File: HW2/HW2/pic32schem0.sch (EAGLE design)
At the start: 21 parts, among them J3 USB-MB-H

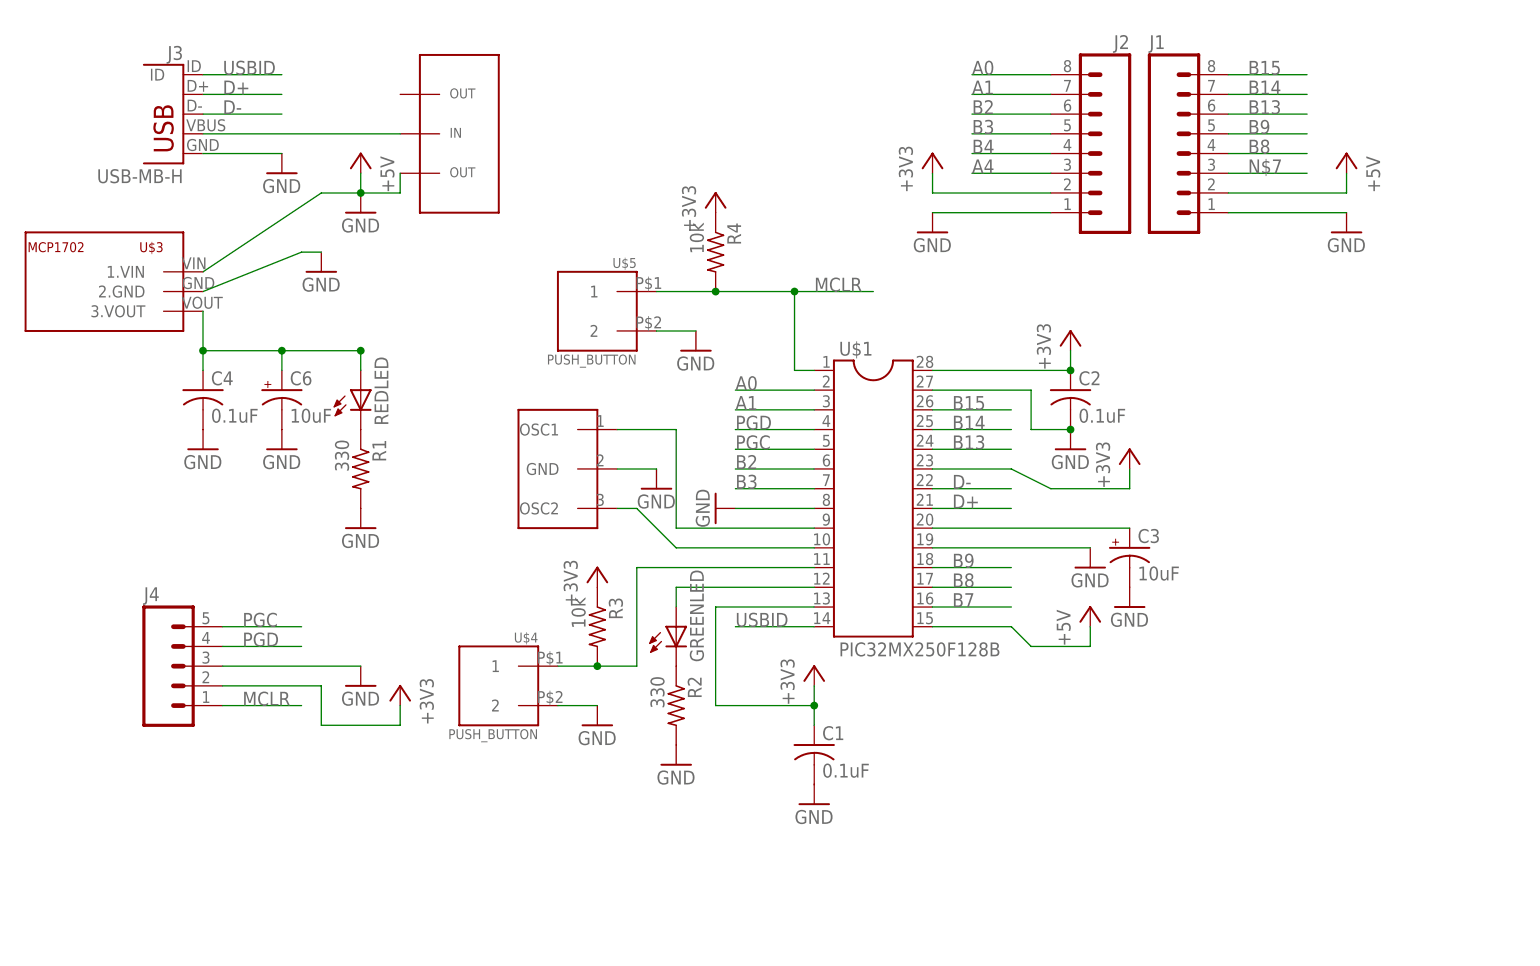
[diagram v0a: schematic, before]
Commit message: Finished pcb, quite a few errors
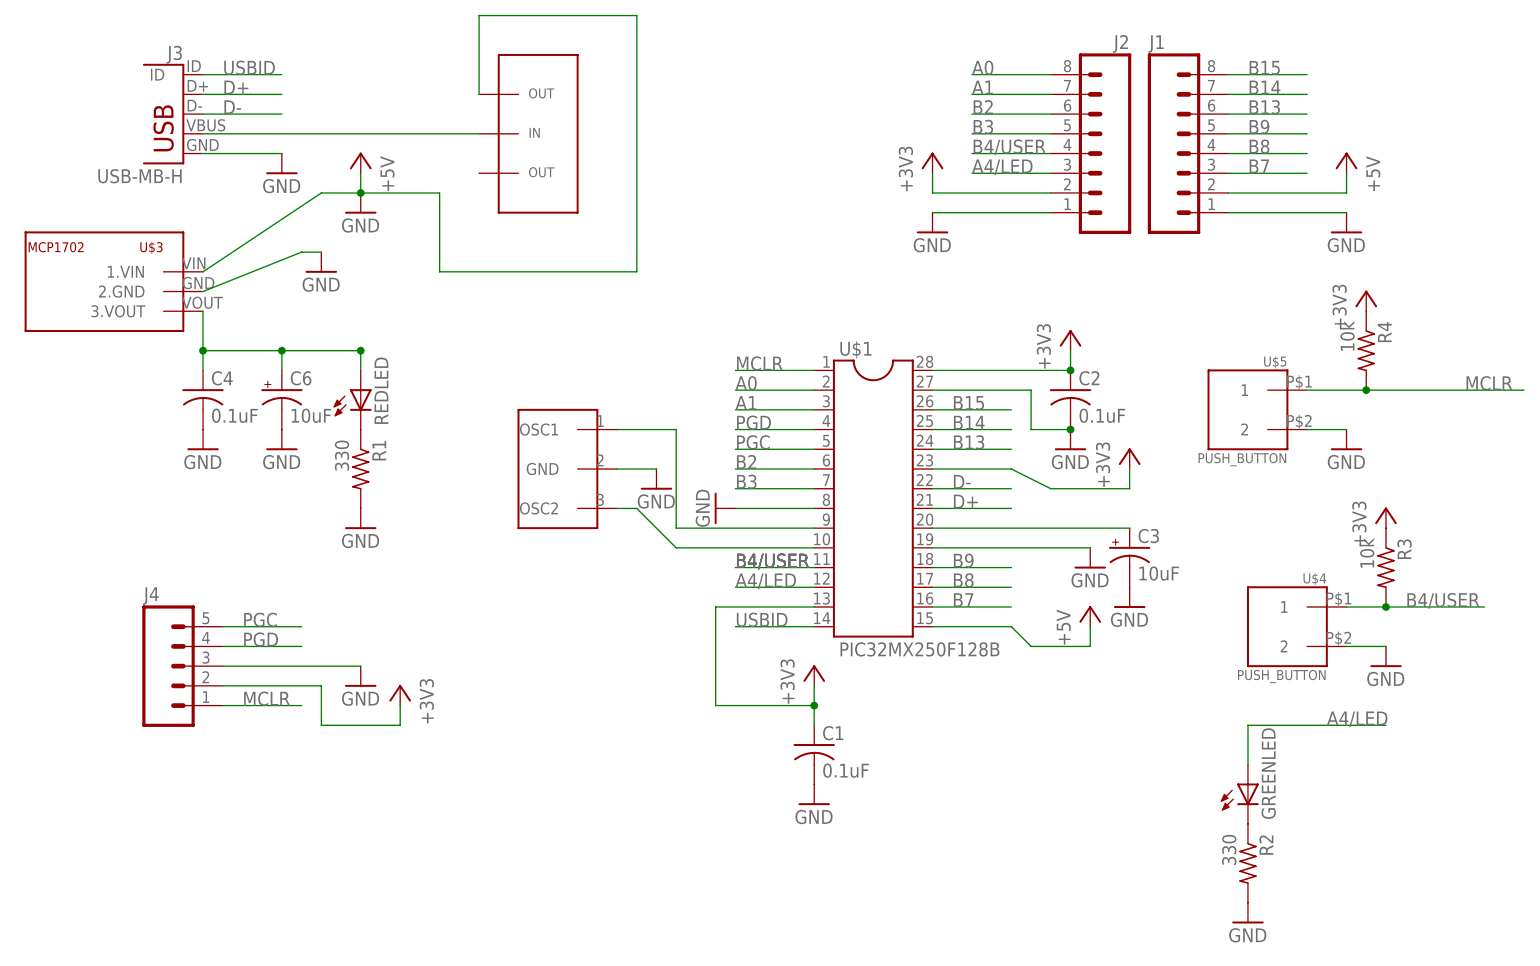
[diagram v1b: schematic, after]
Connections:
- removed net A1/LED: GREENLED.A, U$1.12.SOSCO/RPA4/T1CK/CTED9/PMA1/RA4
- removed net A4: J2.3
- removed net B4: J2.4
- removed net N$7: J1.3
- new net A4/LED: GREENLED.A, J2.3, U$1.12.SOSCO/RPA4/T1CK/CTED9/PMA1/RA4
- net B4/USER: now also J2.4
- net B7: now also J1.3
- net GND: now also U$2.3.OUT; no longer U$2.1.OUT
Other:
- moved on the sheet: GREENLED, R2, R3, R4, U$4, U$5
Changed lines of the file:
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@@
 <part name="REDLED" library="MechE_433" deviceset="LED" device="3MM"/>
 <part name="R1" library="MechE_433" deviceset="R-US_" device="0207/10" value="330"/>
-<part name="GND14" library="MechE_433" deviceset="GND" device=""/>
 <part name="GREENLED" library="MechE_433" deviceset="LED" device="3MM"/>
 <part name="R2" library="MechE_433" deviceset="R-US_" device="0207/10" value="330"/>
@@
 <part name="C6" library="MechE_433" deviceset="CPOL-US" device="B45181A" value="10uF"/>
 <part name="C3" library="MechE_433" deviceset="CPOL-US" device="B45181A" value="10uF"/>
+<part name="GND14" library="MechE_433" deviceset="GND" device=""/>
 </parts>
 <sheets>
@@
 <instance part="+3V4" gate="G$1" x="5.08" y="104.14"/>
 <instance part="GND9" gate="1" x="-78.74" y="101.6"/>
-<instance part="U$2" gate="G$1" x="-60.96" y="106.68"/>
+<instance part="U$2" gate="G$1" x="-50.8" y="106.68"/>
 <instance part="U$3" gate="G$1" x="-91.44" y="86.36" rot="MR0"/>
 <instance part="P+3" gate="1" x="-68.58" y="104.14" rot="MR0"/>
@@
 <instance part="REDLED" gate="G$1" x="-68.58" y="73.66"/>
 <instance part="R1" gate="G$1" x="-68.58" y="63.5" rot="R270"/>
-<instance part="GND14" gate="1" x="-68.58" y="55.88"/>
-<instance part="GREENLED" gate="G$1" x="-27.94" y="43.18"/>
-<instance part="R2" gate="G$1" x="-27.94" y="33.02" rot="R270"/>
-<instance part="GND15" gate="1" x="-27.94" y="25.4"/>
-<instance part="R3" gate="G$1" x="-38.1" y="43.18" rot="R270"/>
-<instance part="+3V5" gate="G$1" x="-38.1" y="50.8"/>
-<instance part="GND16" gate="1" x="-38.1" y="30.48"/>
-<instance part="U$5" gate="G$1" x="-30.48" y="83.82" rot="MR0"/>
-<instance part="R4" gate="G$1" x="-22.86" y="91.44" rot="R270"/>
-<instance part="+3V6" gate="G$1" x="-22.86" y="99.06"/>
-<instance part="GND17" gate="1" x="-25.4" y="78.74"/>
+<instance part="GREENLED" gate="G$1" x="45.72" y="22.86"/>
+<instance part="R2" gate="G$1" x="45.72" y="12.7" rot="R270"/>
+<instance part="GND15" gate="1" x="45.72" y="5.08"/>
+<instance part="R3" gate="G$1" x="63.5" y="50.8" rot="R270"/>
+<instance part="+3V5" gate="G$1" x="63.5" y="58.42"/>
+<instance part="GND16" gate="1" x="63.5" y="38.1"/>
+<instance part="U$5" gate="G$1" x="53.34" y="71.12" rot="MR0"/>
+<instance part="R4" gate="G$1" x="60.96" y="78.74" rot="R270"/>
+<instance part="+3V6" gate="G$1" x="60.96" y="86.36"/>
+<instance part="GND17" gate="1" x="58.42" y="66.04"/>
 <instance part="J4" gate="G$1" x="-93.98" y="38.1"/>
 <instance part="GND18" gate="1" x="-68.58" y="35.56"/>
 <instance part="+3V7" gate="G$1" x="-63.5" y="35.56" rot="MR0"/>
-<instance part="U$4" gate="G$1" x="-43.18" y="35.56" rot="MR0"/>
+<instance part="U$4" gate="G$1" x="58.42" y="43.18" rot="MR0"/>
 <instance part="J3" gate="G$1" x="-91.44" y="104.14" rot="MR0"/>
 <instance part="C6" gate="G$1" x="-78.74" y="73.66"/>
 <instance part="C3" gate="G$1" x="30.48" y="53.34"/>
+<instance part="GND14" gate="1" x="-68.58" y="55.88"/>
 </instances>
 <busses>
@@
 </segment>
 <segment>
-<pinref part="U$2" gate="G$1" pin="1.OUT"/>
-<wire x1="-63.5" y1="101.6" x2="-63.5" y2="99.06" width="0.1524" layer="91"/>
-<wire x1="-63.5" y1="99.06" x2="-68.58" y2="99.06" width="0.1524" layer="91"/>
 <pinref part="U$3" gate="G$1" pin="1.VIN"/>
 <wire x1="-68.58" y1="99.06" x2="-73.66" y2="99.06" width="0.1524" layer="91"/>
@@
 <wire x1="-68.58" y1="101.6" x2="-68.58" y2="99.06" width="0.1524" layer="91"/>
 <pinref part="GND10" gate="1" pin="GND"/>
+<pinref part="U$2" gate="G$1" pin="3.OUT"/>
+<wire x1="-53.34" y1="111.76" x2="-53.34" y2="121.92" width="0.1524" layer="91"/>
+<wire x1="-53.34" y1="121.92" x2="-33.02" y2="121.92" width="0.1524" layer="91"/>
+<wire x1="-33.02" y1="121.92" x2="-33.02" y2="88.9" width="0.1524" layer="91"/>
+<wire x1="-33.02" y1="88.9" x2="-58.42" y2="88.9" width="0.1524" layer="91"/>
+<wire x1="-58.42" y1="88.9" x2="-58.42" y2="99.06" width="0.1524" layer="91"/>
+<wire x1="-58.42" y1="99.06" x2="-68.58" y2="99.06" width="0.1524" layer="91"/>
 </segment>
 <segment>
@@
 </segment>
 <segment>
-<pinref part="R1" gate="G$1" pin="2"/>
-<pinref part="GND14" gate="1" pin="GND"/>
-</segment>
-<segment>
 <pinref part="R2" gate="G$1" pin="2"/>
 <pinref part="GND15" gate="1" pin="GND"/>
 </segment>
 <segment>
-<wire x1="-43.18" y1="33.02" x2="-38.1" y2="33.02" width="0.1524" layer="91"/>
+<wire x1="58.42" y1="40.64" x2="63.5" y2="40.64" width="0.1524" layer="91"/>
 <pinref part="GND16" gate="1" pin="GND"/>
 <pinref part="U$4" gate="G$1" pin="2"/>
@@
 <segment>
 <pinref part="U$5" gate="G$1" pin="2"/>
-<wire x1="-30.48" y1="81.28" x2="-25.4" y2="81.28" width="0.1524" layer="91"/>
+<wire x1="53.34" y1="68.58" x2="58.42" y2="68.58" width="0.1524" layer="91"/>
 <pinref part="GND17" gate="1" pin="GND"/>
 </segment>
@@
 <pinref part="C3" gate="G$1" pin="-"/>
 </segment>
+<segment>
+<pinref part="R1" gate="G$1" pin="2"/>
+<pinref part="GND14" gate="1" pin="GND"/>
+</segment>
 </net>
 <net name="USBID" class="0">
@@
 </segment>
 </net>
-<net name="A1/LED" class="0">
-<segment>
-<pinref part="U$1" gate="G$1" pin="12.SOSCO/RPA4/T1CK/CTED9/PMA1/RA4"/>
-<wire x1="-10.16" y1="48.26" x2="-27.94" y2="48.26" width="0.1524" layer="91"/>
-<wire x1="-27.94" y1="48.26" x2="-27.94" y2="45.72" width="0.1524" layer="91"/>
-<pinref part="GREENLED" gate="G$1" pin="A"/>
-</segment>
-</net>
 <net name="B4/USER" class="0">
 <segment>
-<pinref part="U$1" gate="G$1" pin="11.SOSCI/RPB4/RB4"/>
-<wire x1="-10.16" y1="50.8" x2="-33.02" y2="50.8" width="0.1524" layer="91"/>
-<wire x1="-33.02" y1="50.8" x2="-33.02" y2="38.1" width="0.1524" layer="91"/>
-<wire x1="-33.02" y1="38.1" x2="-38.1" y2="38.1" width="0.1524" layer="91"/>
-<junction x="-38.1" y="38.1"/>
-<wire x1="-38.1" y1="38.1" x2="-43.18" y2="38.1" width="0.1524" layer="91"/>
+<wire x1="76.2" y1="45.72" x2="63.5" y2="45.72" width="0.1524" layer="91"/>
+<junction x="63.5" y="45.72"/>
+<wire x1="63.5" y1="45.72" x2="58.42" y2="45.72" width="0.1524" layer="91"/>
 <pinref part="R3" gate="G$1" pin="2"/>
 <pinref part="U$4" gate="G$1" pin="1"/>
+<label x="66.04" y="45.72" size="1.778" layer="95"/>
+</segment>
+<segment>
+<pinref part="J2" gate="G$1" pin="4"/>
+<wire x1="20.32" y1="104.14" x2="10.16" y2="104.14" width="0.1524" layer="91"/>
+<label x="10.16" y="104.14" size="1.778" layer="95"/>
+</segment>
+<segment>
+<pinref part="U$1" gate="G$1" pin="11.SOSCI/RPB4/RB4"/>
+<wire x1="-10.16" y1="50.8" x2="-20.32" y2="50.8" width="0.1524" layer="91"/>
+<label x="-20.32" y="50.8" size="1.778" layer="95"/>
+<label x="-20.32" y="50.8" size="1.778" layer="95"/>
+<label x="-20.32" y="50.8" size="1.778" layer="95"/>
 </segment>
 </net>
@@
 <wire x1="5.08" y1="45.72" x2="15.24" y2="45.72" width="0.1524" layer="91"/>
 <label x="7.62" y="45.72" size="1.778" layer="95"/>
+</segment>
+<segment>
+<pinref part="J1" gate="G$1" pin="3"/>
+<wire x1="43.18" y1="101.6" x2="53.34" y2="101.6" width="0.1524" layer="91"/>
+<label x="45.72" y="101.6" size="1.778" layer="95"/>
 </segment>
 </net>
@@
 </segment>
 </net>
-<net name="N$7" class="0">
-<segment>
-<pinref part="J1" gate="G$1" pin="3"/>
-<wire x1="43.18" y1="101.6" x2="53.34" y2="101.6" width="0.1524" layer="91"/>
-<label x="45.72" y="101.6" size="1.778" layer="95"/>
-</segment>
-</net>
-<net name="B4" class="0">
-<segment>
-<pinref part="J2" gate="G$1" pin="4"/>
-<wire x1="20.32" y1="104.14" x2="10.16" y2="104.14" width="0.1524" layer="91"/>
-<label x="10.16" y="104.14" size="1.778" layer="95"/>
-</segment>
-</net>
-<net name="A4" class="0">
+<net name="A4/LED" class="0">
 <segment>
 <pinref part="J2" gate="G$1" pin="3"/>
 <wire x1="20.32" y1="101.6" x2="10.16" y2="101.6" width="0.1524" layer="91"/>
 <label x="10.16" y="101.6" size="1.778" layer="95"/>
+</segment>
+<segment>
+<pinref part="GREENLED" gate="G$1" pin="A"/>
+<wire x1="45.72" y1="25.4" x2="45.72" y2="30.48" width="0.1524" layer="91"/>
+<wire x1="45.72" y1="30.48" x2="63.5" y2="30.48" width="0.1524" layer="91"/>
+<label x="55.88" y="30.48" size="1.778" layer="95"/>
+</segment>
+<segment>
+<pinref part="U$1" gate="G$1" pin="12.SOSCO/RPA4/T1CK/CTED9/PMA1/RA4"/>
+<wire x1="-10.16" y1="48.26" x2="-20.32" y2="48.26" width="0.1524" layer="91"/>
+<label x="-20.32" y="48.26" size="1.778" layer="95"/>
 </segment>
 </net>
@@
 </segment>
 <segment>
+<pinref part="U$5" gate="G$1" pin="1"/>
+<pinref part="R4" gate="G$1" pin="2"/>
+<wire x1="60.96" y1="73.66" x2="53.34" y2="73.66" width="0.1524" layer="91"/>
+<junction x="60.96" y="73.66"/>
+<wire x1="60.96" y1="73.66" x2="81.28" y2="73.66" width="0.1524" layer="91"/>
+<label x="73.66" y="73.66" size="1.778" layer="95"/>
+</segment>
+<segment>
 <pinref part="U$1" gate="G$1" pin="1.MCLR_BAR"/>
-<wire x1="-10.16" y1="76.2" x2="-12.7" y2="76.2" width="0.1524" layer="91"/>
-<wire x1="-12.7" y1="76.2" x2="-12.7" y2="86.36" width="0.1524" layer="91"/>
-<pinref part="U$5" gate="G$1" pin="1"/>
-<wire x1="-12.7" y1="86.36" x2="-22.86" y2="86.36" width="0.1524" layer="91"/>
-<pinref part="R4" gate="G$1" pin="2"/>
-<wire x1="-22.86" y1="86.36" x2="-30.48" y2="86.36" width="0.1524" layer="91"/>
-<junction x="-22.86" y="86.36"/>
-<wire x1="-12.7" y1="86.36" x2="-2.54" y2="86.36" width="0.1524" layer="91"/>
-<junction x="-12.7" y="86.36"/>
-<label x="-10.16" y="86.36" size="1.778" layer="95"/>
-</segment>
-</net>
-<net name="N$12" class="0">
+<wire x1="-10.16" y1="76.2" x2="-20.32" y2="76.2" width="0.1524" layer="91"/>
+<label x="-20.32" y="76.2" size="1.778" layer="95"/>
+</segment>
+</net>
+<net name="N$5" class="0">
 <segment>
 <pinref part="J3" gate="G$1" pin="VBUS"/>
 <pinref part="U$2" gate="G$1" pin="2.IN"/>
-<wire x1="-88.9" y1="106.68" x2="-63.5" y2="106.68" width="0.1524" layer="91"/>
-</segment>
-</net>
+<wire x1="-88.9" y1="106.68" x2="-53.34" y2="106.68" width="0.1524" layer="91"/>
+</segment>
+</net>
